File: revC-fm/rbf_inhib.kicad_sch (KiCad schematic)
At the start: 12 parts, among them Q2 MMDT5551-7-F, Q21 MMDT3946, Q22 BSZ180P03NS3GATMA1, Q23 BSZ180P03NS3GATMA1

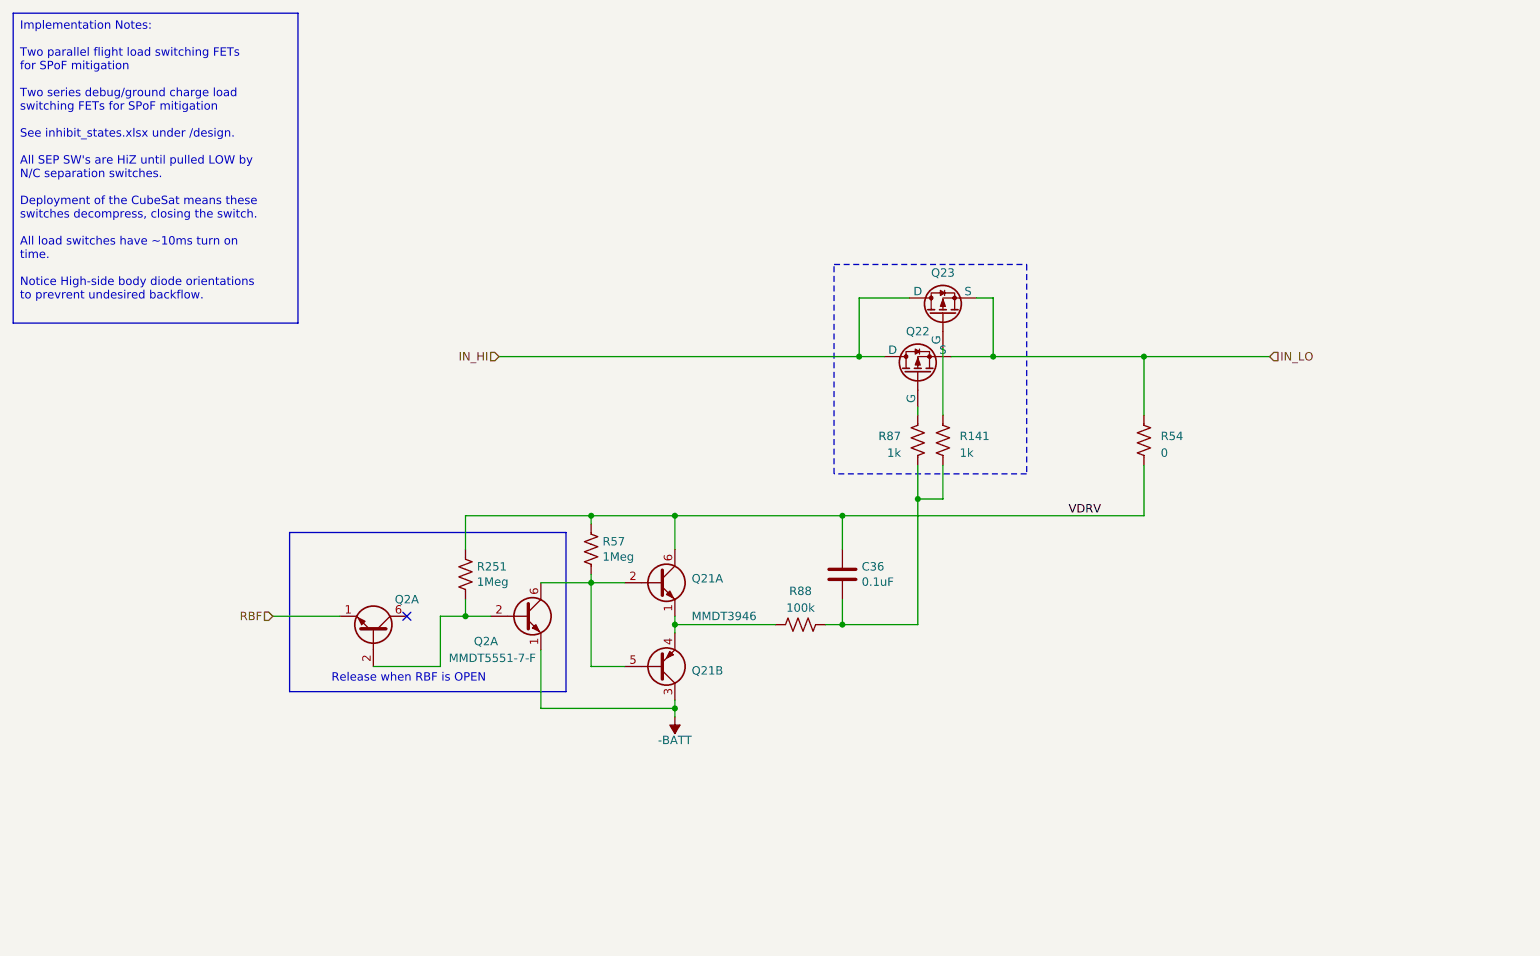
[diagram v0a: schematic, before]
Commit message: almost done!!!!!
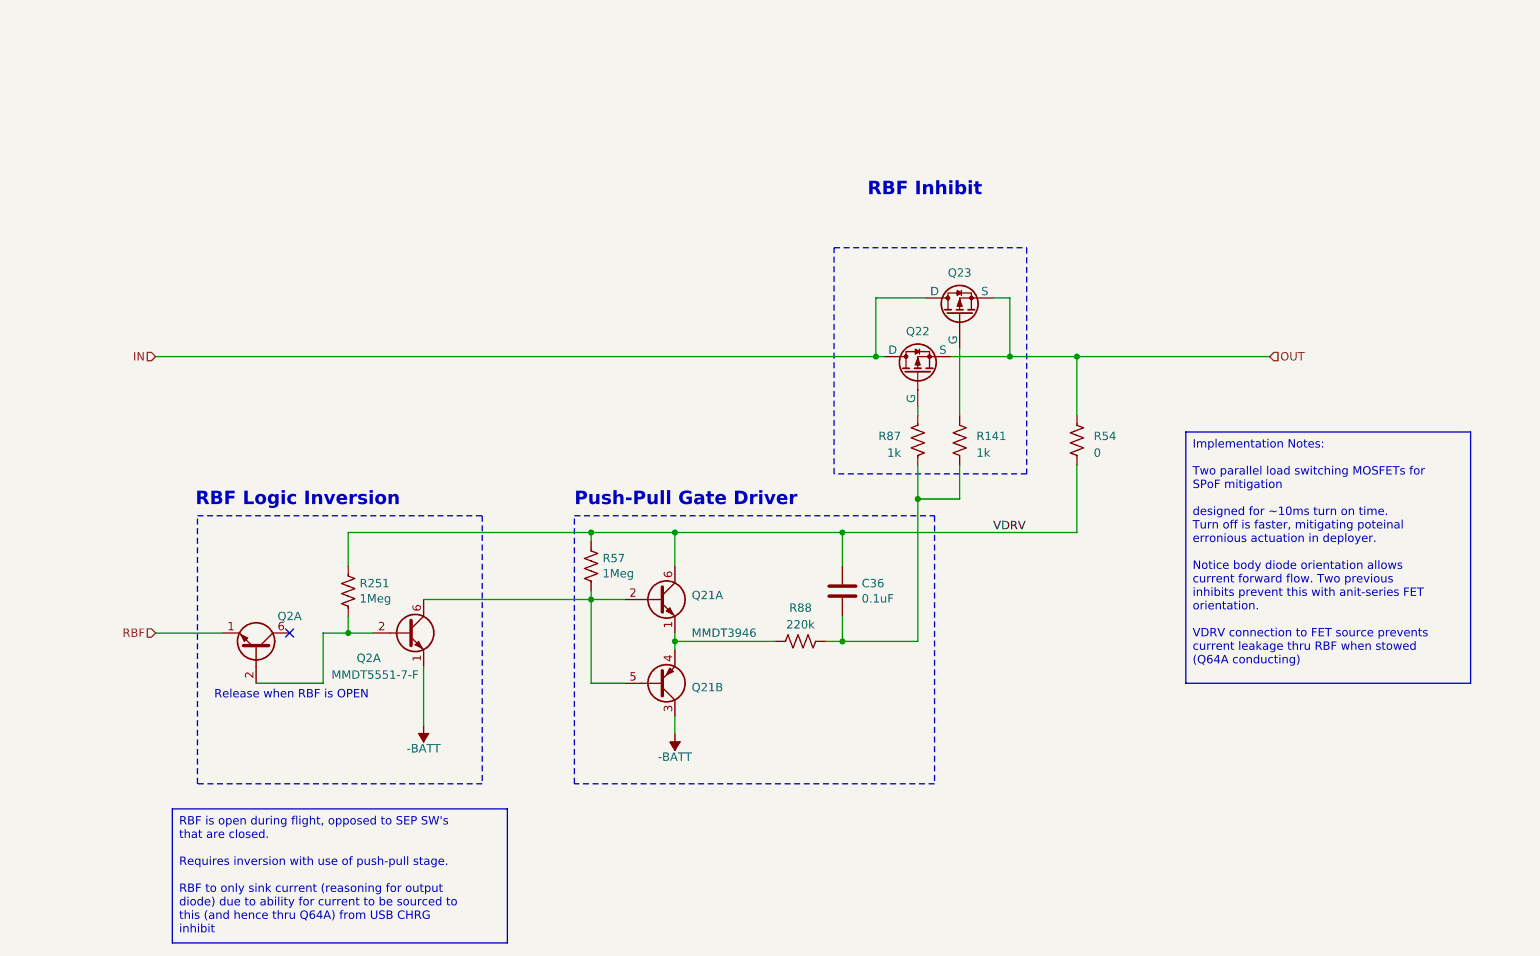
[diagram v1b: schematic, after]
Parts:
- Q22, Q23: value BSZ180P03NS3GATMA1 -> BSZ180
- R88: value 100k -> 220k
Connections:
- net IN_HI renamed IN
- net IN_LO renamed OUT
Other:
- note added: "Push-Pull Gate Driver"
- note added: "RBF Inhibit"
- note added: "RBF Logic Inversion"
- moved on the sheet: C36, Q21A, Q21B, Q23, Q2A, R141, R251, R54, R57, R88

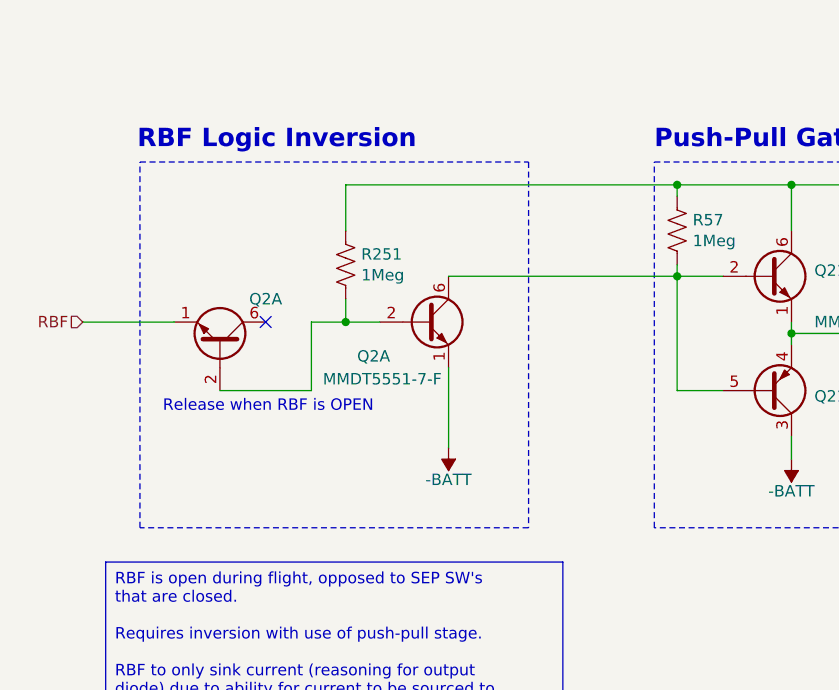
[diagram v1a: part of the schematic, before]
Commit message: updated fab files
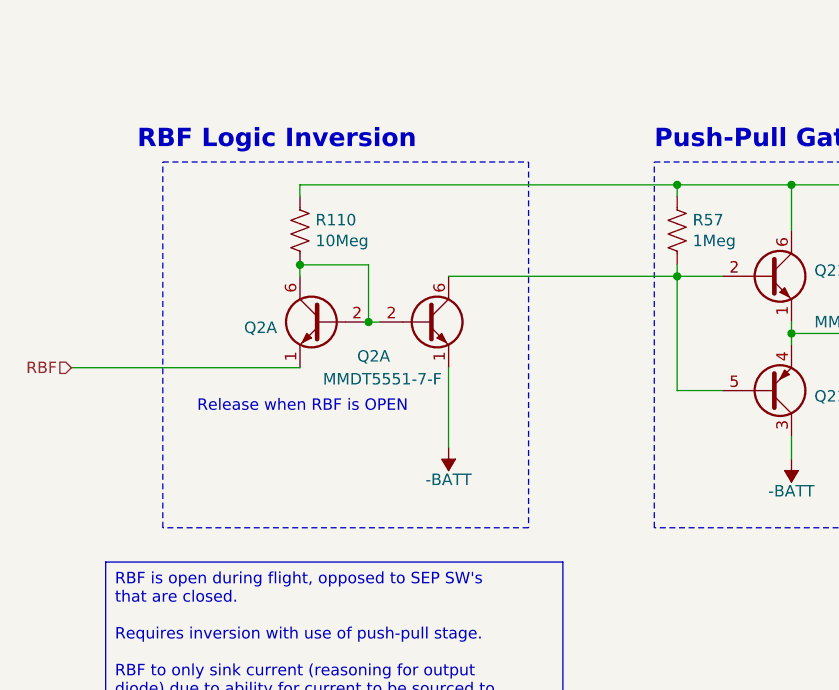
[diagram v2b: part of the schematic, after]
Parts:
- C36: Manufacturer (none) -> TDK; Mfr. Part No (none) -> CGA2B3X7R1H104K050BE
- Q2: Manufacturer (none) -> Diodes Incorporated; Mfr. Part No (none) -> MMDT5551-7-F
- Q21: Manufacturer (none) -> Diodes Incorporated
- Q22, Q23: Manufacturer (none) -> Infineon
- R110: renamed from R251; value 1Meg -> 10Meg; Manufacturer (none) -> Stackpole Electronics; Mfr. Part No (none) -> RMCF0402FT10M0
- R141, R87: Manufacturer (none) -> Panasonic; Mfr. Part No (none) -> ERJ-2GEJ102X
- R54: Manufacturer (none) -> Stackpole Electronics; Mfr. Part No (none) -> RMCF0603ZT0R00
- R57: Manufacturer (none) -> Stackpole Electronics; Mfr. Part No (none) -> RMCF0402FT1M00
- R88: Manufacturer (none) -> Stackpole Electronics; Mfr. Part No (none) -> RMCF0402FT220K
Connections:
- net at Q2.2 (B1), Q2.2 (B1), R110.2: now also Q2.6 (C1)
- no-connect marks 1 -> 0
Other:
- moved on the sheet: Q2A, R110
